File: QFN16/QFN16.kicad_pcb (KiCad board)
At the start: 2 copper layers, 20.6 x 13 mm, 9 parts, among them J1 Conn_01x08, J2 Conn_02x08_Counter_Clockwise, J3 Conn_01x08, J4 Conn_02x08_Counter_Clockwise, J5 Conn_01x03

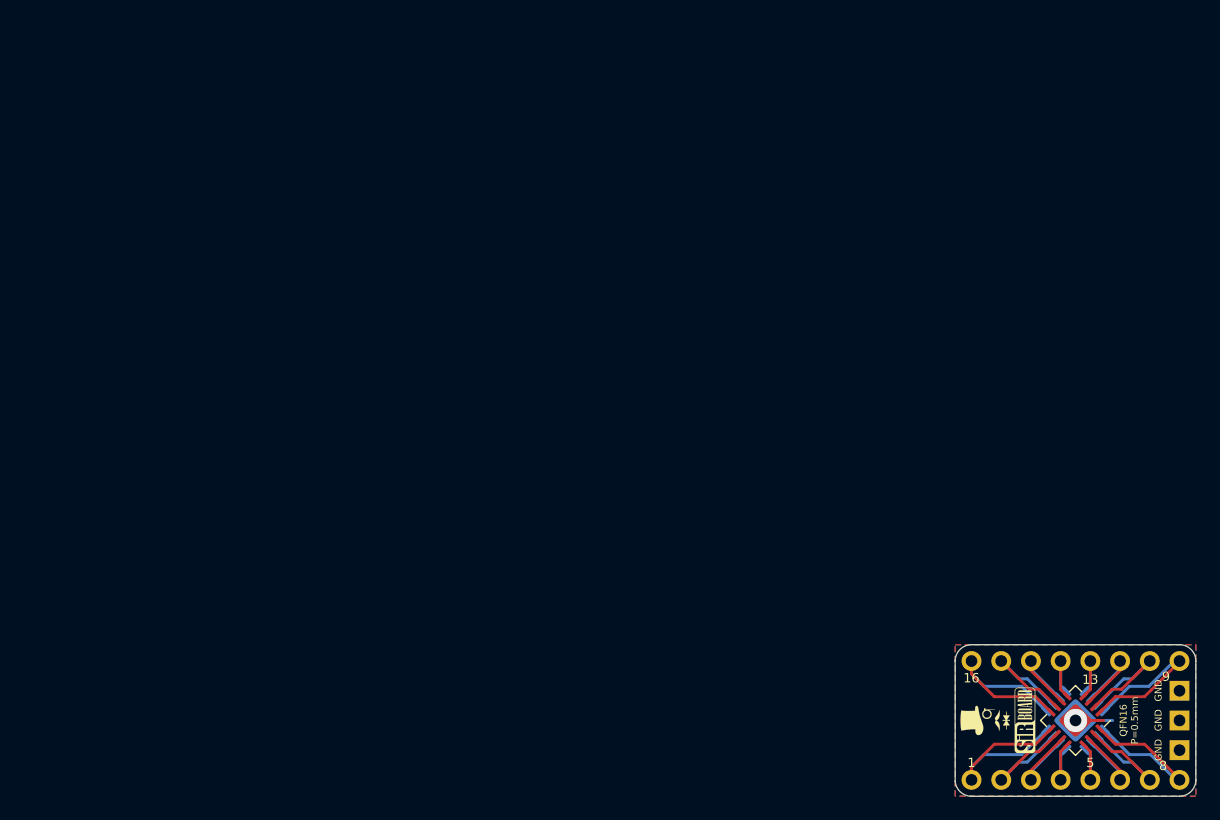
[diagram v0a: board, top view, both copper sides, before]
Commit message: Page Settings Updated
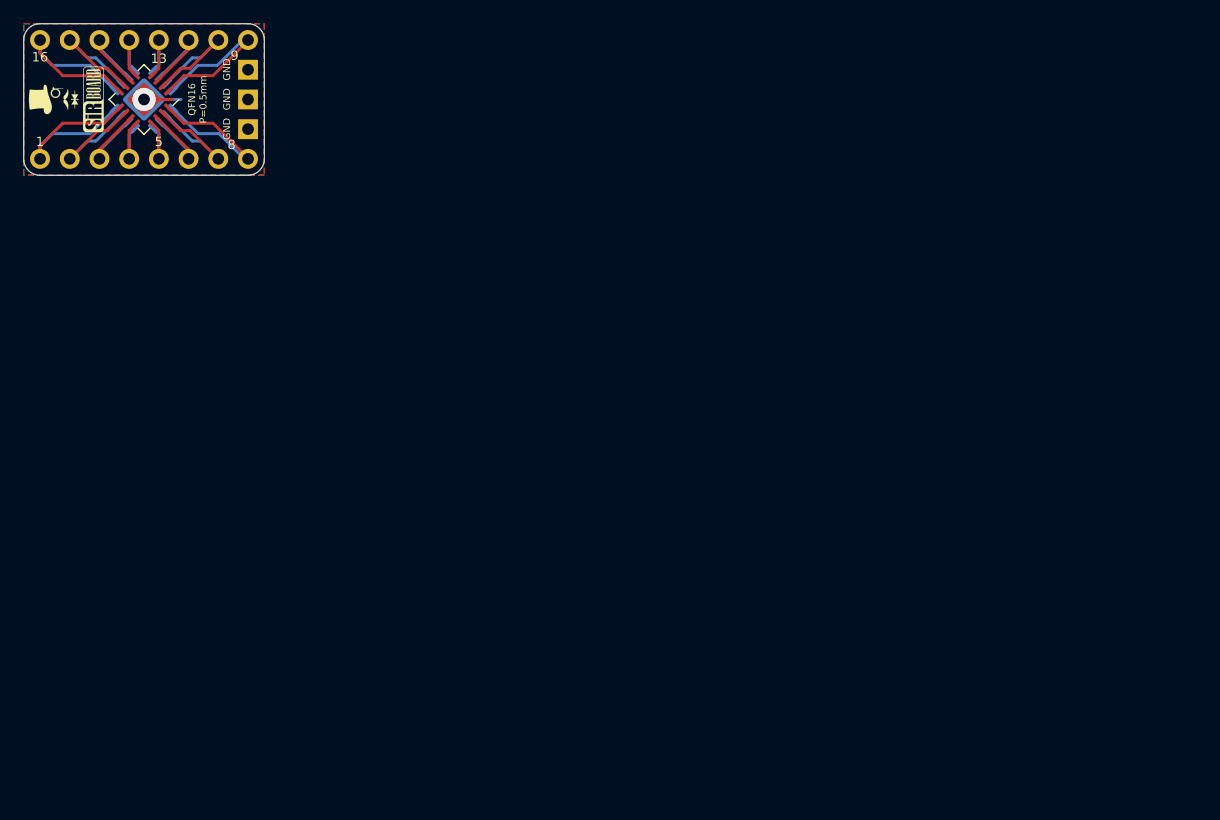
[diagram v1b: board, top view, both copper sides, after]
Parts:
- moved G*** 95.7 mm to (65.5, 41.0)
- moved J2 95.7 mm to (70.4, 41.0)
- moved J4 95.7 mm to (70.4, 41.0)
- moved G*** 95.7 mm to (62.4, 41.0)
- moved G*** 95.7 mm to (66.0, 41.0)
- moved G*** 95.7 mm to (62.6, 41.0)
- moved J1 95.7 mm to (79.3, 35.9)
- moved J3 95.7 mm to (79.3, 46.0)
- moved J5 95.7 mm to (79.3, 38.4)
